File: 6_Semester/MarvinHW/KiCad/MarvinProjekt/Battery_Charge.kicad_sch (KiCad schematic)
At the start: 13 parts, among them U5 DW01A, U6 FS8205A, U7 HM4056H

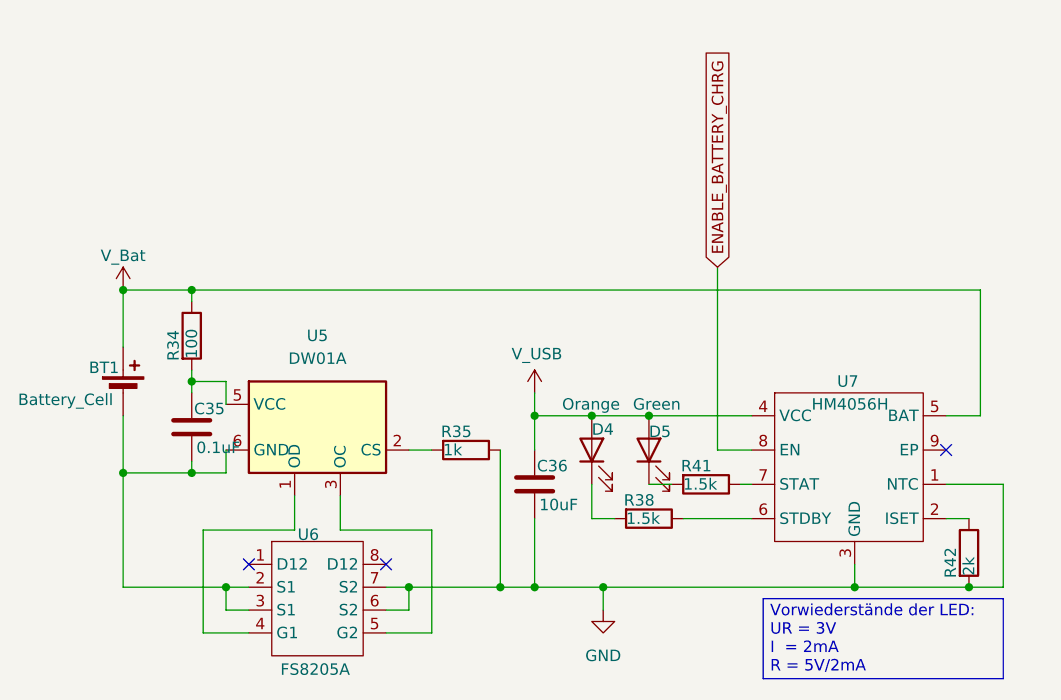
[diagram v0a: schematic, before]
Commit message: finish evaluat components
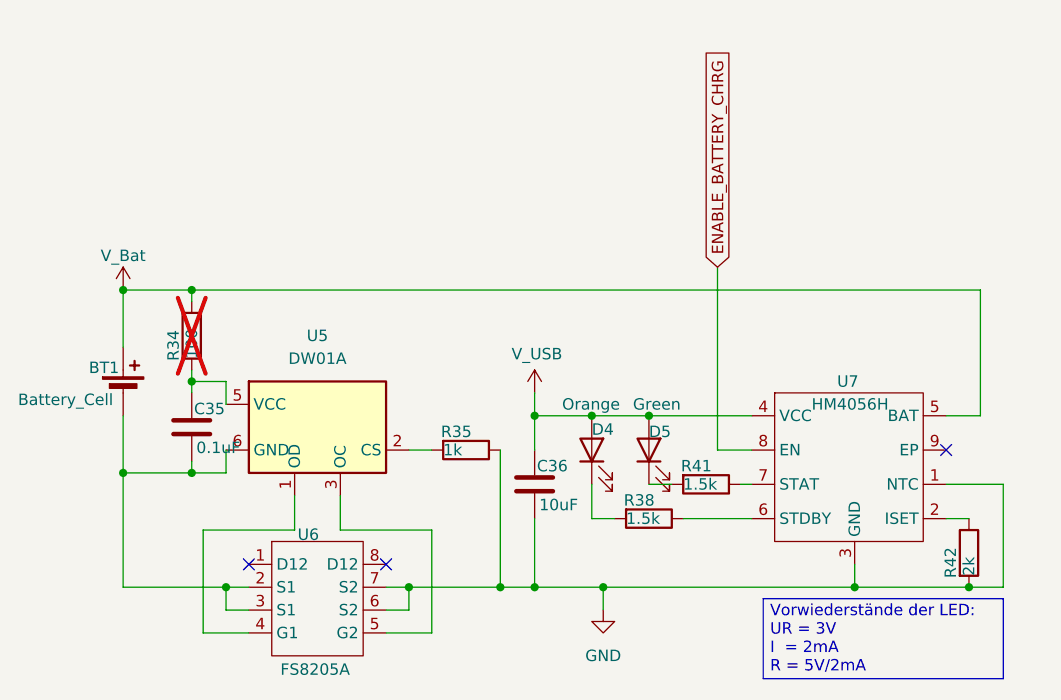
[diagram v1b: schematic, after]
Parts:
- R34: now not fitted
- U7: LCSC Part (none) -> C16581
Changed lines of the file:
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@@
 		(in_bom yes)
 		(on_board yes)
-		(dnp no)
+		(dnp yes)
 		(property "Reference" "R34"
 			(at 103.378 85.344 90)
@@
 			(at 179.07 96.52 0)
 			(effects
+				(font
+					(size 1.27 1.27)
+				)
+				(hide yes)
+			)
+		)
+		(property "LCSC Part" "C16581"
+			(at 179.07 96.52 0)
+			(effects
